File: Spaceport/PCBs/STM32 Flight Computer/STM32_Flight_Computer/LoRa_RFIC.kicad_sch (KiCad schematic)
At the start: 1 part, among them U8 SX1273IMLTRT

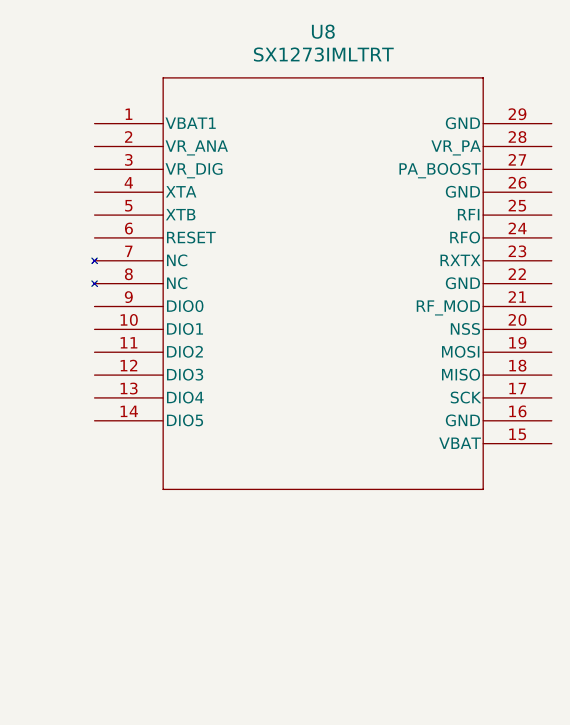
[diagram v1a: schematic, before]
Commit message: Push
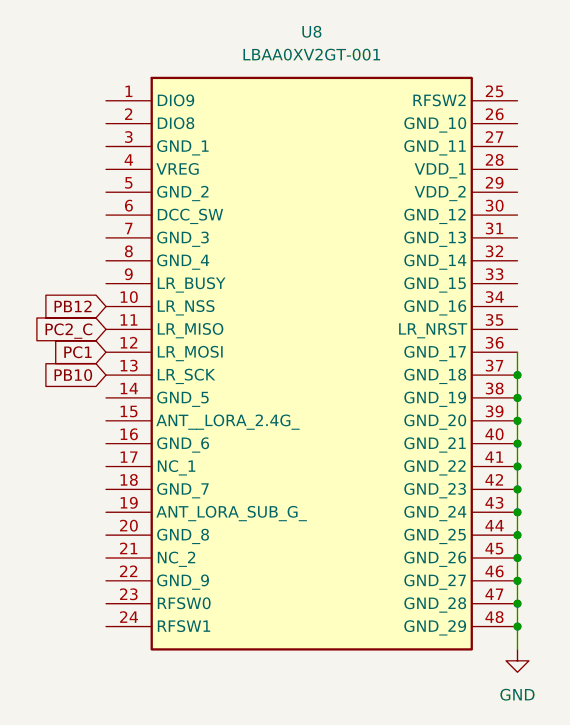
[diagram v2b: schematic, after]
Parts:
- removed U8: SX1273IMLTRT, QFN28_SEM, symbol SRAD_AVIONICS:SX1273IMLTRT
- added U8: LBAA0XV2GT-001, LBAA0XV2GT001, symbol SRAD_AVIONICS:LBAA0XV2GT-001
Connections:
- new net GND: U8.36 (GND_17), U8.37 (GND_18), U8.38 (GND_19), U8.39 (GND_20), U8.40 (GND_21), U8.41 (GND_22), U8.42 (GND_23), U8.43 (GND_24), U8.44 (GND_25), U8.45 (GND_26), U8.46 (GND_27), U8.47 (GND_28), U8.48 (GND_29)
- new net PB10: U8.13 (LR_SCK)
- new net PB12: U8.10 (LR_NSS)
- new net PC1: U8.12 (LR_MOSI)
- new net PC2_C: U8.11 (LR_MISO)

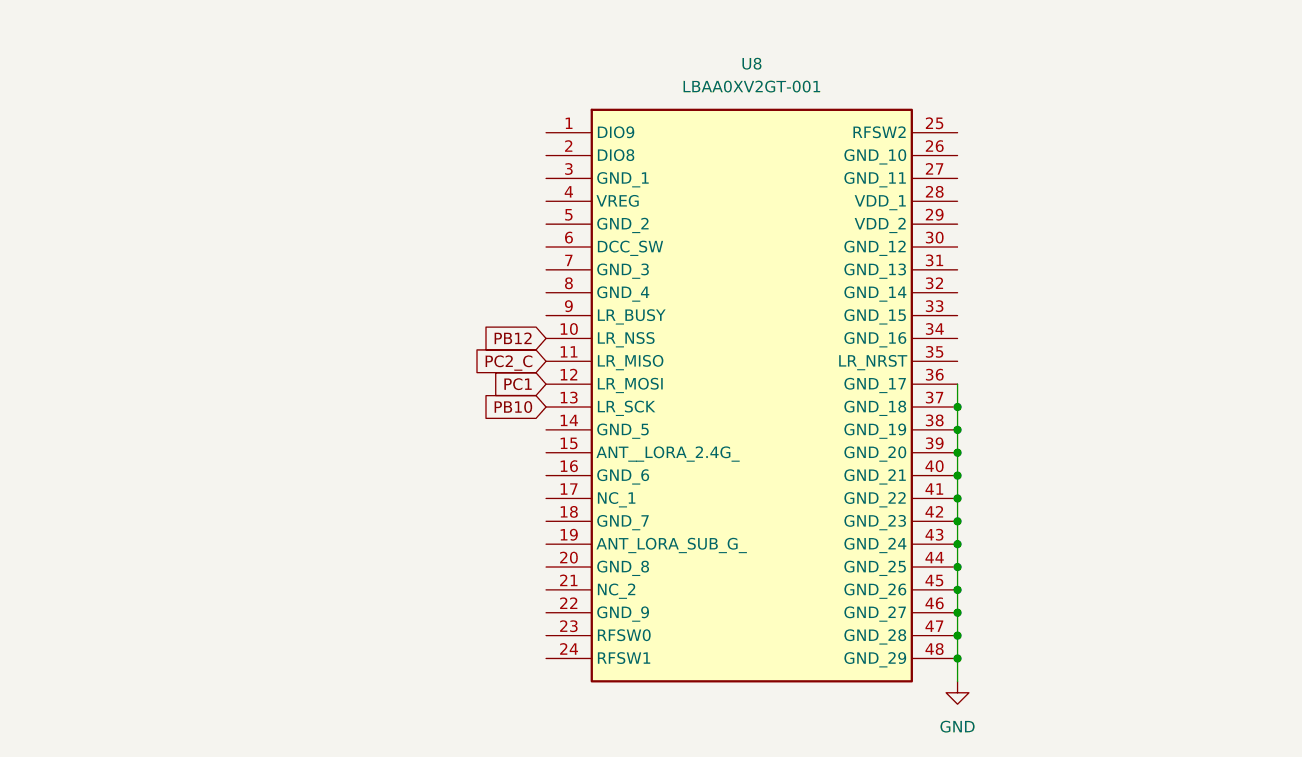
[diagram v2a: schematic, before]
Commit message: Push after Schematic Review 5/5
- Updated STM32 symbol
- Configured I2C busses
- Updated DC caps to 100nF
- TODO add power system things
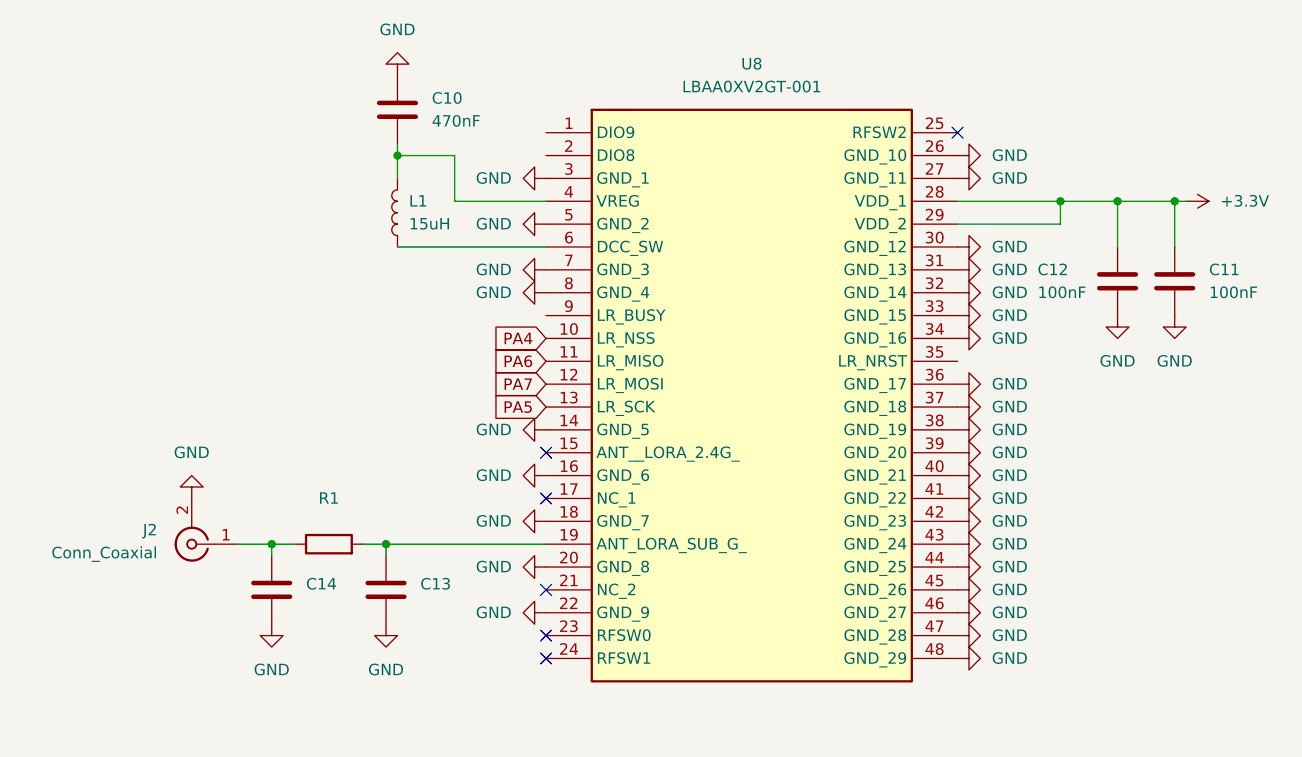
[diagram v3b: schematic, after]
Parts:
- added C10: 470nF, symbol Device:C
- added C11, C12: 100nF, symbol Device:C
- added C13, C14: ~, symbol Device:C
- added J2: Conn_Coaxial, symbol Connector:Conn_Coaxial
- added L1: 15uH, symbol Device:L
- added R1: ~, symbol Device:R
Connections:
- net GND: now also U8.14 (GND_5), U8.16 (GND_6), U8.18 (GND_7), U8.20 (GND_8), U8.22 (GND_9), U8.26 (GND_10), U8.27 (GND_11), U8.3 (GND_1), U8.30 (GND_12), U8.31 (GND_13), U8.32 (GND_14), U8.33 (GND_15), U8.34 (GND_16), U8.5 (GND_2), U8.7 (GND_3), U8.8 (GND_4), C10.1, C11.1, C12.1, C13.1, C14.1, J2.2 (Ext)
- net at U8.19 (ANT_LORA_SUB_G_): now also C13.2, R1.2
- net +3.3V: now reaches U8.28 (VDD_1)
- net +3.3V: now also U8.29 (VDD_2), C11.2, C12.2
- net at U8.4 (VREG): now also C10.2, L1.2
- net at U8.6 (DCC_SW): now also L1.1
- net PB10 renamed PA5
- net PB12 renamed PA4
- net PC1 renamed PA7
- net PC2_C renamed PA6
- new net: C14.2, J2.1 (In), R1.1
- no-connect marks 0 -> 6
